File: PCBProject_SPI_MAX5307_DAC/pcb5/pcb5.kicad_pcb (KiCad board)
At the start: 4 copper layers, 93.9 x 51.7 mm, 80 parts, among them IC1 MAX5725BAUP+, U1 SN74HC365D, U2 LM224DR, U3 LM224DR

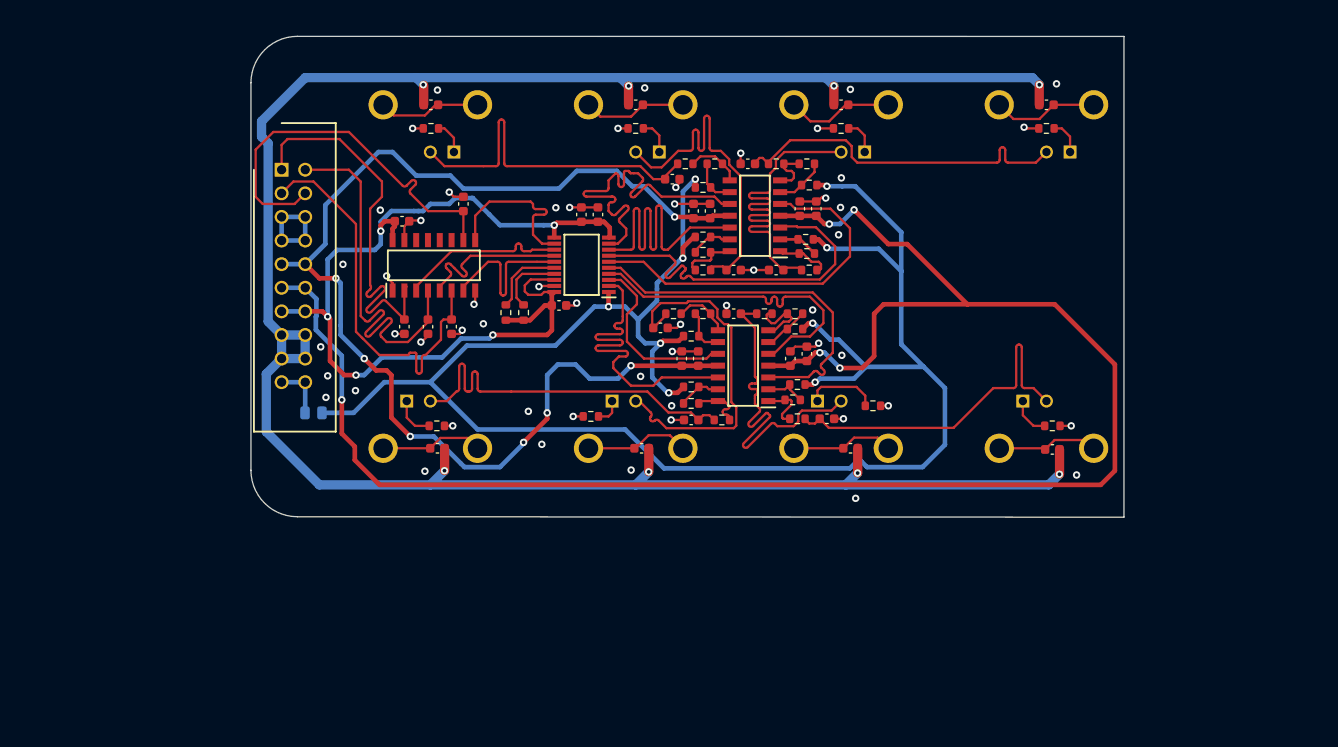
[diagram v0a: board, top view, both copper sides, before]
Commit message: DAC for 28388
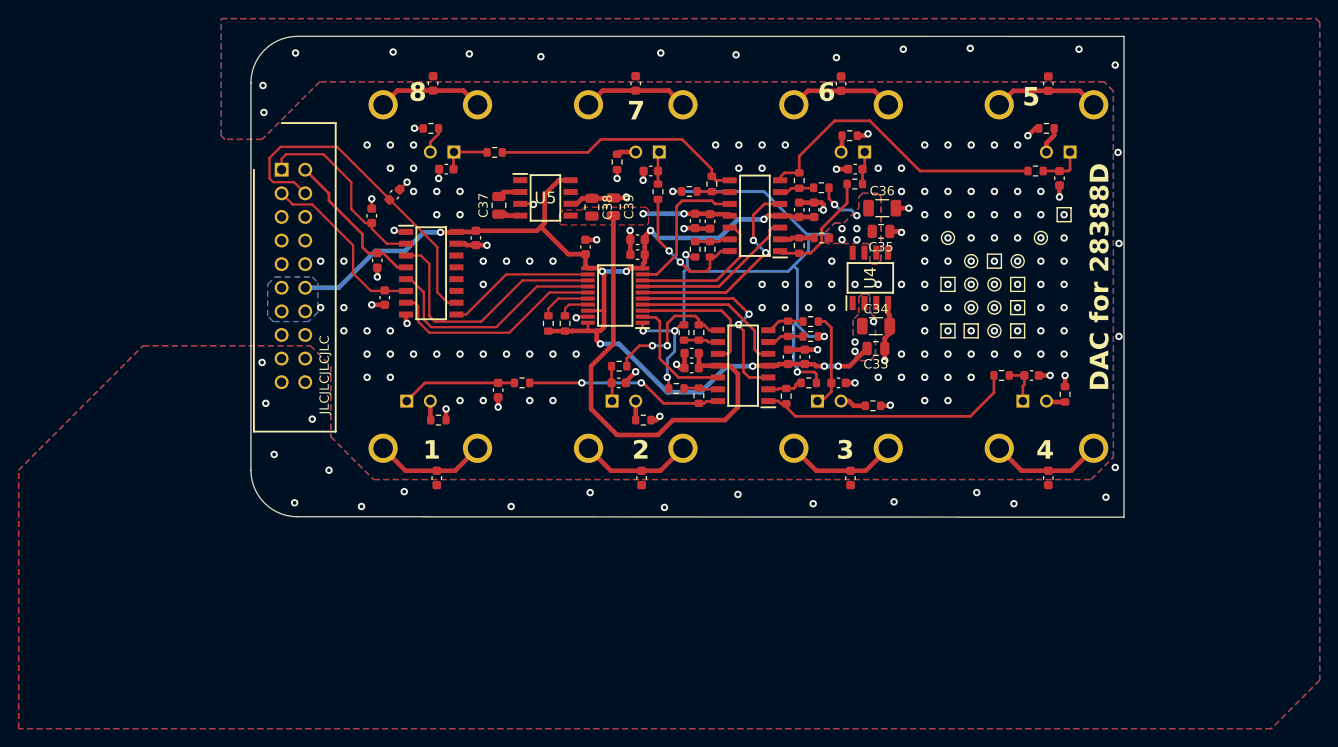
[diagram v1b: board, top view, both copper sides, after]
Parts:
- removed RU1: 0R, Resistor_SMD:R_0805_2012Metric
- added C33: 104, Capacitor_SMD:C_0805_2012Metric, F.Cu at (122.0, 81.3)
- added C34: 106 25V, Capacitor_SMD:C_1206_3216Metric, F.Cu at (122.0, 78.9)
- added C35: 104, Capacitor_SMD:C_0805_2012Metric, F.Cu at (122.5, 68.7)
- added C36: 106 25V, Capacitor_SMD:C_1206_3216Metric, F.Cu at (122.7, 66.2)
- added C37: 10uF, Capacitor_SMD:C_0805_2012Metric, F.Cu at (81.4, 65.9)
- added C38: 10uF, Capacitor_SMD:C_0805_2012Metric, F.Cu at (91.4, 66.1)
- added C39: 0.1uF, Capacitor_SMD:C_0805_2012Metric, F.Cu at (93.7, 66.1)
- added G***: LOGO, LOGO, B.Cu at (125.2, 73.9)
- added U4: ADR423ARZ, SamacSys_Parts:SOIC127P600X175-8N, F.Cu at (121.4, 73.7)
- added U5: LM2662M_NOPB, SamacSys_Parts:SOIC127P600X175-8N, F.Cu at (86.4, 65.1)
- moved C26 33.6 mm to (141.7, 63.0), turned to -90 degrees
- moved R19 27.9 mm to (139.2, 62.2), turned to 0 degrees
- moved C30 24.3 mm to (75.8, 62.0), turned to 180 degrees
- moved C23 22.5 mm to (138.7, 84.2)
- moved R13 22.5 mm to (135.5, 84.2)
- moved R34 21.9 mm to (83.9, 85.0)
- moved C32 21.0 mm to (81.3, 85.8), turned to -90 degrees
- moved R28 20.5 mm to (81.0, 60.2)
- moved C31 13.9 mm to (97.8, 62.2), turned to 180 degrees
- moved C24 13.8 mm to (119.8, 62.0)
- moved C27 13.5 mm to (118.0, 85.0), turned to 0 degrees
- moved C1 12.4 mm to (67.7, 67.1), turned to 90 degrees
- moved R14 10.5 mm to (119.7, 63.6), turned to 0 degrees
- moved R33 9.72 mm to (98.5, 64.5), turned to 90 degrees
- moved C2 8.97 mm to (68.3, 71.9)
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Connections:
- net /SPISIMIA_5V renamed /SPISOMIA_5V
- net /SPI_C_CK_HS renamed /SPI_CK_HS
- net /SPI_C_MI_HS renamed /SPI_MI_HS
- net /SPI_C_MO_HS renamed /SPI_MO_HS
- net /~{SPI_C_STE_HS} renamed /~{SPI_STE_HS}
- BNC1 pad 1: Net-(BNC1-Pad1) -> /DACA
- BNC1 pad 2: /DACA -> Net-(BNC1-Pad2)
- BNC2 pad 1: Net-(BNC2-Pad1) -> /DACB
- BNC2 pad 2: /DACB -> Net-(BNC2-Pad2)
- BNC3 pad 1: Net-(BNC3-Pad1) -> /DACC
- BNC3 pad 2: /DACC -> Net-(BNC3-Pad2)
- BNC4 pad 1: Net-(BNC4-Pad1) -> /DACD
- BNC4 pad 2: /DACD -> Net-(BNC4-Pad2)
- BNC5 pad 1: Net-(BNC5-Pad1) -> /DACE
- BNC5 pad 2: /DACE -> Net-(BNC5-Pad2)
- BNC6 pad 1: Net-(BNC6-Pad1) -> /DACF
- BNC6 pad 2: /DACF -> Net-(BNC6-Pad2)
- BNC7 pad 1: Net-(BNC7-Pad1) -> /DACG
- BNC7 pad 2: /DACG -> Net-(BNC7-Pad2)
- BNC8 pad 1: Net-(BNC8-Pad1) -> /DACH
- BNC8 pad 2: /DACH -> Net-(BNC8-Pad2)
- C14 pad 1: -5V_ADC -> -5V
- C15 pad 2: -5V_ADC -> -5V
- C16 pad 1: -5V_ADC -> -5V
- C17 pad 2: -5V_ADC -> -5V
- C18 pad 1: A+5V -> D+5V
- C19 pad 1: A+5V -> D+5V
- C20 pad 2: A+5V -> D+5V
- C21 pad 2: A+5V -> D+5V
- R1 pad 2: Net-(BNC1-Pad1) -> Net-(BNC1-Pad2)
- R2 pad 2: Net-(BNC5-Pad1) -> Net-(BNC5-Pad2)
- R3 pad 2: Net-(BNC2-Pad1) -> Net-(BNC2-Pad2)
- R4 pad 2: Net-(BNC6-Pad1) -> Net-(BNC6-Pad2)
- R5 pad 2: Net-(BNC3-Pad1) -> Net-(BNC3-Pad2)
- R6 pad 2: Net-(BNC7-Pad1) -> Net-(BNC7-Pad2)
- R7 pad 2: Net-(BNC4-Pad1) -> Net-(BNC4-Pad2)
- R8 pad 2: Net-(BNC8-Pad1) -> Net-(BNC8-Pad2)
- SPI-DAC1 pad 10: -5V_ADC -> unconnected-(SPI-DAC1-Pad10)
- SPI-DAC1 pad 11: A+5V -> D+5V
- SPI-DAC1 pad 12: A+5V -> D+5V
- SPI-DAC1 pad 15: PE_GND -> unconnected-(SPI-DAC1-Pad15)
- SPI-DAC1 pad 16: PE_GND -> unconnected-(SPI-DAC1-Pad16)
- SPI-DAC1 pad 19: Net-(RU1-Pad2) -> PE_GND
- SPI-DAC1 pad 20: Net-(RU1-Pad2) -> PE_GND
- SPI-DAC1 pad 9: -5V_ADC -> unconnected-(SPI-DAC1-Pad9)
- U2 pad 11: -5V_ADC -> -5V
- U2 pad 4: A+5V -> D+5V
- U3 pad 11: -5V_ADC -> -5V
- U3 pad 4: A+5V -> D+5V
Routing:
- net PE_GND: track 245.0 -> 0.00 mm, vias 8 -> 34
- net A+5V: track 190.4 -> 0.00 mm, vias 5 -> 0
- net -5V_ADC: track 128.8 -> 0.00 mm, vias 7 -> 0
- net REF_3V: track 208.8 -> 85.2 mm, vias 9 -> 13
- net -5V: track 0.00 -> 59.2 mm, vias 0 -> 2
- net /DACB: track 38.4 -> 3.78 mm
- net /DACG: track 38.1 -> 3.50 mm
- net /DACF: track 38.0 -> 3.54 mm
- net /DACD: track 38.0 -> 4.45 mm
- net /DACE: track 38.0 -> 4.85 mm
- net /DACH: track 38.2 -> 5.44 mm
- net /DACA: track 41.8 -> 12.4 mm
- net /DACC: track 37.6 -> 10.5 mm
- net Net-(R17-Pad2): track 5.97 -> 32.8 mm
- net /SPI_CK_HS: track 43.1 -> 16.5 mm
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- added copper zone on F.Cu, net -5V
- added copper zone on B.Cu, net D+5V
- added copper zone on F.Cu, net D+5V
- added copper zone on B.Cu, net PE_GND
- added copper zone on F.Cu, net PE_GND
- added copper zone on In1.Cu, net PE_GND
- added copper zone on In2.Cu, net PE_GND
- added copper zone on B.Cu, net REF_3V
- added copper zone on F.Cu, net REF_3V
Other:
- board text added: "1"
- board text added: "2"
- board text added: "3"
- board text added: "4"
- board text added: "5"
- board text added: "6"
- board text added: "7"
- board text added: "8"
- board text added: "DAC for 28388D"
- board text added: "JLCJLCJLCJLC"
- board text added: "Meow"
